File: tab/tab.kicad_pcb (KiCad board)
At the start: 2 copper layers, 29 x 17.8 mm, 14 parts

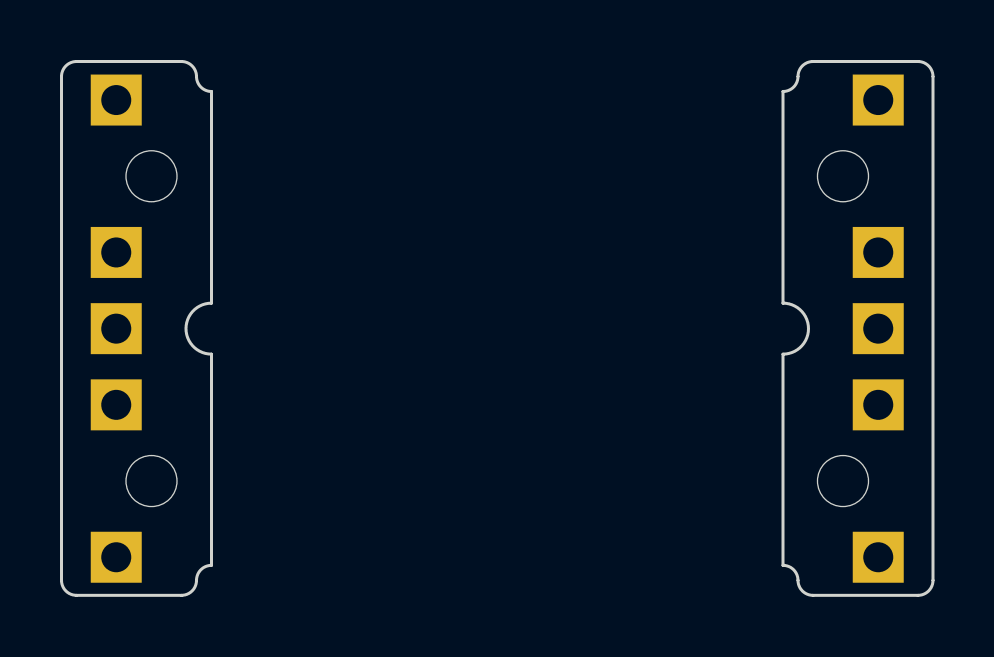
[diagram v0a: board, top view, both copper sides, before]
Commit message: make symmetric
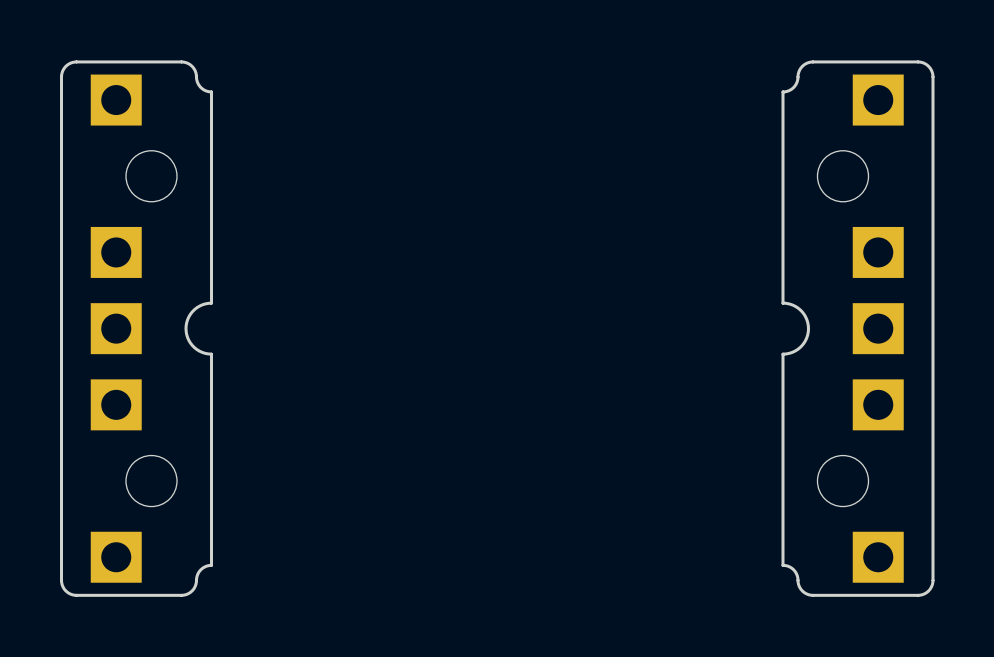
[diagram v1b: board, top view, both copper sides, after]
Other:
- outline, holes or cut-outs redrawn
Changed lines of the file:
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@@
     (pad "1" thru_hole rect (at 0 0 180) (size 1.7 1.7) (drill 1) (layers "*.Cu" "*.Mask"))
   )
-  (gr_arc (start 83.455 69.835) (mid 83.808553 69.981447) (end 83.955 70.335)
+  (gr_arc (start 83.455 69.85) (mid 83.808553 69.996447) (end 83.955 70.35)
     (stroke (width 0.1) (type default)) (layer "Edge.Cuts"))
-  (gr_line (start 83.455 69.835) (end 79.955 69.835)
+  (gr_line (start 83.455 69.85) (end 79.955 69.85)
     (stroke (width 0.1) (type default)) (layer "Edge.Cuts"))
-  (gr_arc (start 84.455 70.835) (mid 84.101447 70.688553) (end 83.955 70.335)
+  (gr_arc (start 84.455 70.85) (mid 84.101447 70.703553) (end 83.955 70.35)
     (stroke (width 0.1) (type default)) (layer "Edge.Cuts"))
-  (gr_arc (start 104.005 70.335) (mid 104.151447 69.981447) (end 104.505 69.835)
+  (gr_line (start 108.005 69.85) (end 104.505 69.85)
     (stroke (width 0.1) (type default)) (layer "Edge.Cuts"))
-  (gr_line (start 103.505 77.89) (end 103.505 70.835)
+  (gr_arc (start 104.005 70.35) (mid 104.151447 69.996447) (end 104.505 69.85)
     (stroke (width 0.1) (type default)) (layer "Edge.Cuts"))
-  (gr_arc (start 79.455 70.335) (mid 79.601447 69.981447) (end 79.955 69.835)
+  (gr_line (start 103.505 77.89) (end 103.505 70.85)
+    (stroke (width 0.1) (type default)) (layer "Edge.Cuts"))
+  (gr_arc (start 79.455 70.35) (mid 79.601447 69.996447) (end 79.955 69.85)
     (stroke (width 0.1) (type default)) (layer "Edge.Cuts"))
   (gr_arc (start 83.955 87.13) (mid 83.808553 87.483553) (end 83.455 87.63)
     (stroke (width 0.1) (type default)) (layer "Edge.Cuts"))
-  (gr_line (start 84.455 70.835) (end 84.455 77.89)
+  (gr_line (start 84.455 70.85) (end 84.455 77.89)
     (stroke (width 0.1) (type default)) (layer "Edge.Cuts"))
   (gr_arc (start 103.505 77.89) (mid 104.355 78.74) (end 103.505 79.59)
@@
     (stroke (width 0.1) (type default)) (layer "Edge.Cuts"))
   (gr_line (start 84.455 79.59) (end 84.455 86.63)
-    (stroke (width 0.1) (type default)) (layer "Edge.Cuts"))
-  (gr_line (start 104.505 69.835) (end 108.005 69.835)
     (stroke (width 0.1) (type default)) (layer "Edge.Cuts"))
   (gr_arc (start 79.955 87.63) (mid 79.601447 87.483553) (end 79.455 87.13)
@@
   (gr_line (start 83.455 87.63) (end 79.955 87.63)
     (stroke (width 0.1) (type default)) (layer "Edge.Cuts"))
-  (gr_line (start 79.455 87.13) (end 79.455 70.335)
+  (gr_line (start 79.455 87.13) (end 79.455 70.35)
     (stroke (width 0.1) (type default)) (layer "Edge.Cuts"))
-  (gr_arc (start 104.005 70.335) (mid 103.858553 70.688553) (end 103.505 70.835)
+  (gr_arc (start 104.005 70.35) (mid 103.858553 70.703553) (end 103.505 70.85)
     (stroke (width 0.1) (type default)) (layer "Edge.Cuts"))
   (gr_arc (start 108.505 87.13) (mid 108.358553 87.483553) (end 108.005 87.63)
     (stroke (width 0.1) (type default)) (layer "Edge.Cuts"))
-  (gr_line (start 108.505 70.335) (end 108.505 87.13)
+  (gr_line (start 108.505 70.35) (end 108.505 87.13)
     (stroke (width 0.1) (type default)) (layer "Edge.Cuts"))
   (gr_arc (start 83.955 87.13) (mid 84.101447 86.776447) (end 84.455 86.63)
     (stroke (width 0.1) (type default)) (layer "Edge.Cuts"))
-  (gr_arc (start 108.005 69.835) (mid 108.358553 69.981447) (end 108.505 70.335)
+  (gr_arc (start 108.005 69.85) (mid 108.358553 69.996447) (end 108.505 70.35)
     (stroke (width 0.1) (type default)) (layer "Edge.Cuts"))
   (gr_arc (start 103.505 86.63) (mid 103.858553 86.776447) (end 104.005 87.13)
